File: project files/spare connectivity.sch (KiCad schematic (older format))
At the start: 2 parts, among them J6 Target STDC-14, U3 STM32F103CBUx

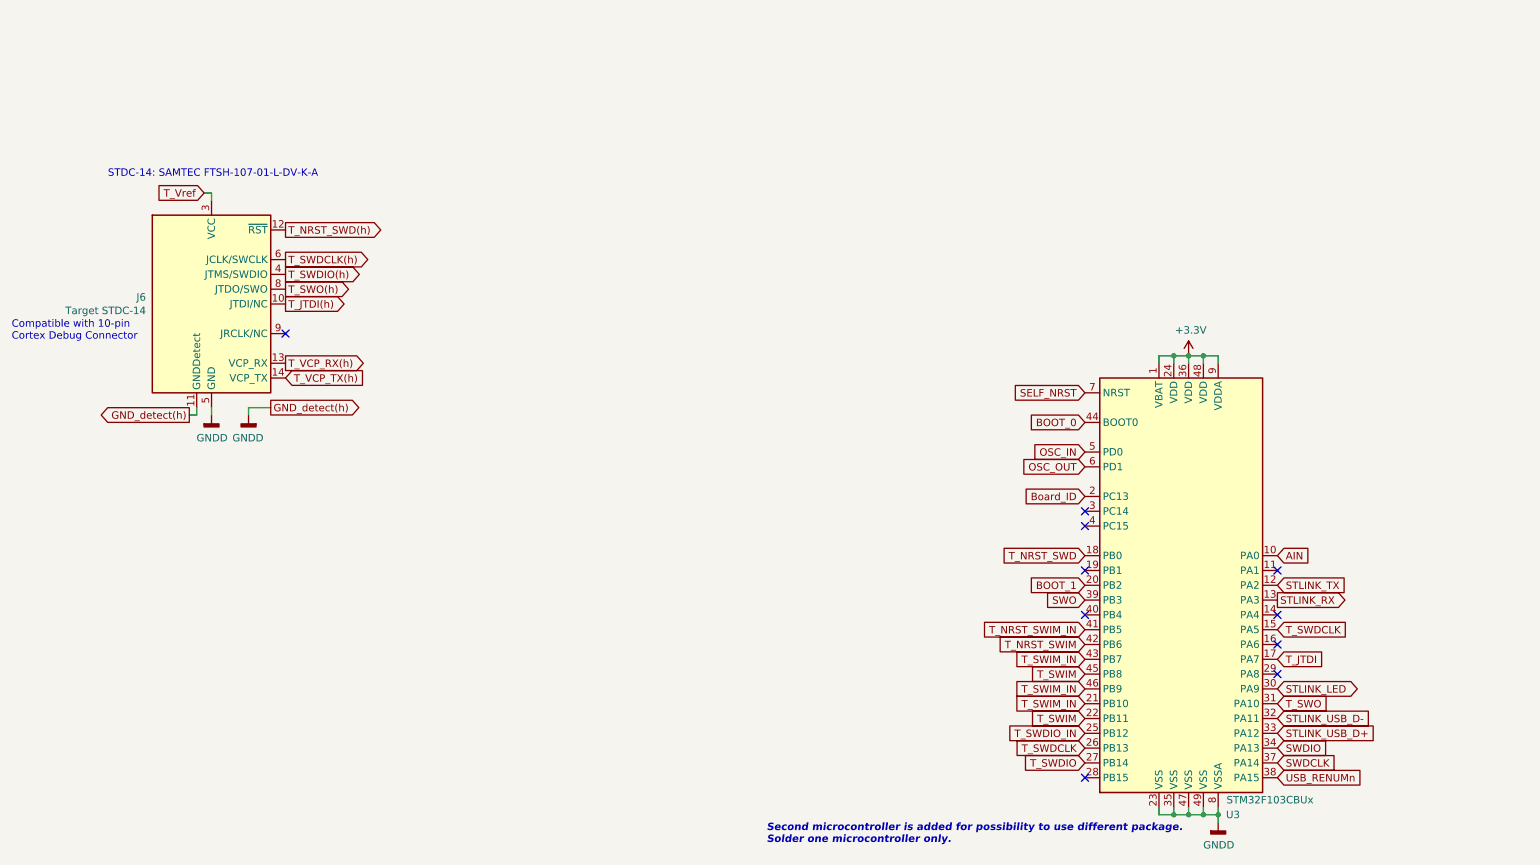
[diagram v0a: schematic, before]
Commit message: fixes
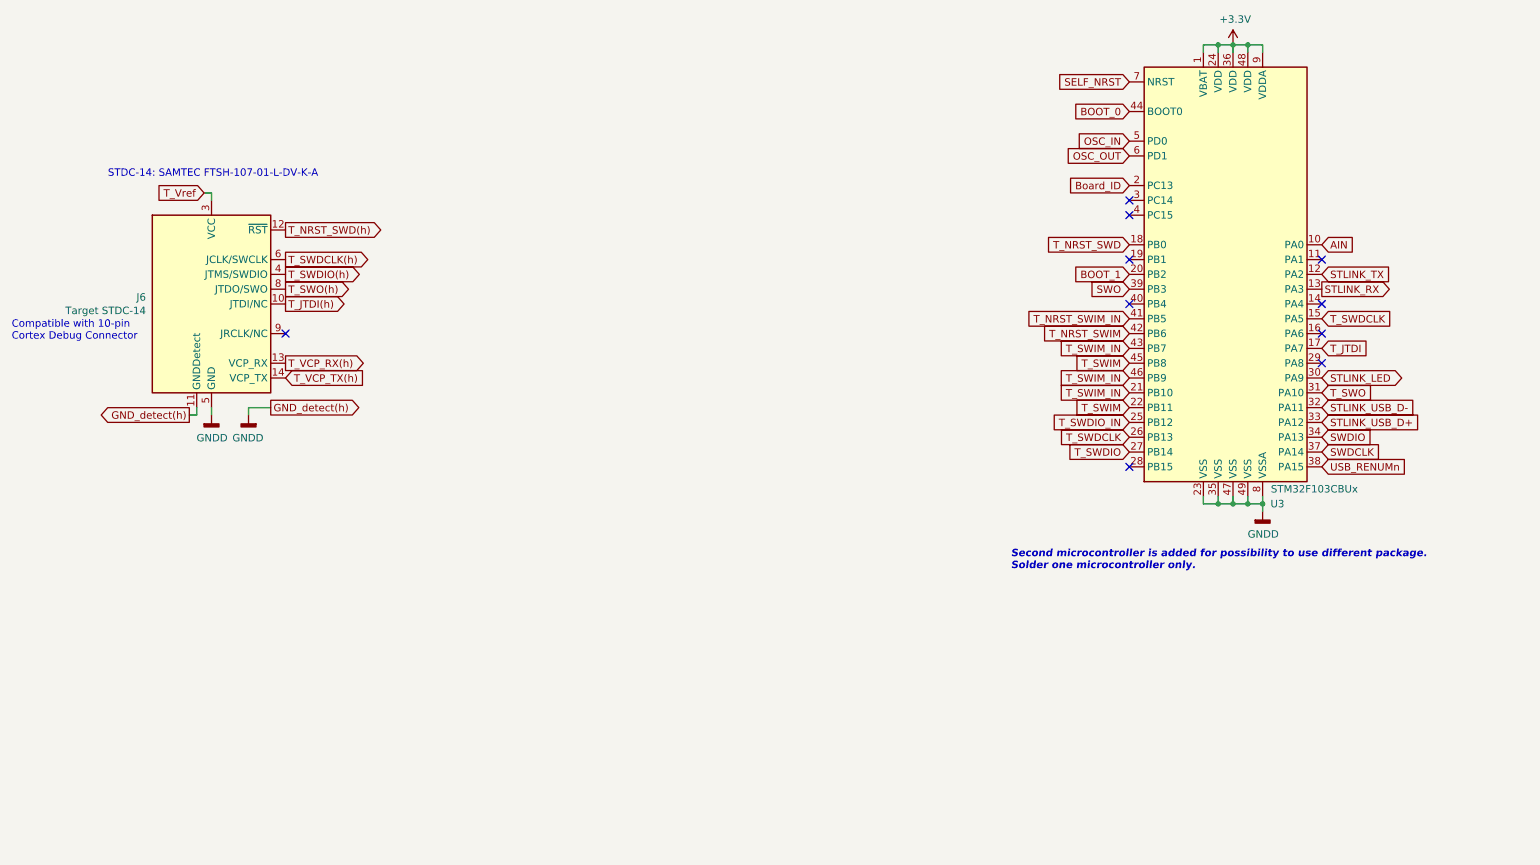
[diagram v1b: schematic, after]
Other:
- moved on the sheet: U3
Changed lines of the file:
@@
 Text Notes 2250 1800 0    50   ~ 0
 STDC-14: SAMTEC FTSH-107-01-L-DV-K-A
-Text GLabel 2800 3400 0    50   Output ~ 0
-GND_detect(h)
-Text GLabel 3350 3350 2    50   Output ~ 0
-GND_detect(h)
 $Comp
 L power:GNDD #PWR?
@@
 T_Vref
 Wire Wire Line
-	9750 6100 9750 6050
-Wire Wire Line
-	9650 6050 9650 6100
-Connection ~ 9650 6100
-Wire Wire Line
-	9650 6100 9750 6100
-Wire Wire Line
-	9550 6050 9550 6100
-Connection ~ 9550 6100
-Wire Wire Line
-	9550 6100 9650 6100
-Wire Wire Line
-	9450 6050 9450 6100
-Connection ~ 9450 6100
-Wire Wire Line
-	9450 6100 9550 6100
-Wire Wire Line
-	9350 6050 9350 6100
-Wire Wire Line
-	9350 6100 9450 6100
+	10050 4000 10050 3950
+Wire Wire Line
+	9950 3950 9950 4000
+Connection ~ 9950 4000
+Wire Wire Line
+	9950 4000 10050 4000
+Wire Wire Line
+	9850 3950 9850 4000
+Connection ~ 9850 4000
+Wire Wire Line
+	9850 4000 9950 4000
+Wire Wire Line
+	9750 3950 9750 4000
+Connection ~ 9750 4000
+Wire Wire Line
+	9750 4000 9850 4000
+Wire Wire Line
+	9650 3950 9650 4000
+Wire Wire Line
+	9650 4000 9750 4000
 $Comp
 L power:GNDD #PWR053
 U 1 1 5EC6BDFB
-P 9750 6150
-F 0 "#PWR053" H 9750 5900 50  0001 C CNN
-F 1 "GNDD" H 9754 5995 50  0000 C CNN
-F 2 "" H 9750 6150 50  0001 C CNN
-F 3 "" H 9750 6150 50  0001 C CNN
-	1    9750 6150
-	1    0    0    -1
-$EndComp
-Wire Wire Line
-	9750 6150 9750 6100
-Connection ~ 9750 6100
-Text Notes 6700 6300 0    50   Italic 10
+P 10050 4050
+F 0 "#PWR053" H 10050 3800 50  0001 C CNN
+F 1 "GNDD" H 10054 3895 50  0000 C CNN
+F 2 "" H 10050 4050 50  0001 C CNN
+F 3 "" H 10050 4050 50  0001 C CNN
+	1    10050 4050
+	1    0    0    -1
+$EndComp
+Wire Wire Line
+	10050 4050 10050 4000
+Connection ~ 10050 4000
+Text Notes 8350 4450 0    50   Italic 10
 Second microcontroller is added for possibility to use different package.\nSolder one microcontroller only.
-NoConn ~ 10150 5150
-NoConn ~ 10150 4950
-NoConn ~ 10150 4750
-NoConn ~ 10150 4450
-NoConn ~ 8850 5850
-NoConn ~ 8850 4750
-NoConn ~ 8850 4450
-NoConn ~ 8850 4150
-NoConn ~ 8850 4050
-Wire Wire Line
-	9350 3050 9350 3000
-Wire Wire Line
-	9450 3050 9450 3000
-Wire Wire Line
-	9550 3050 9550 3000
-Wire Wire Line
-	9650 3050 9650 3000
-Wire Wire Line
-	9750 3050 9750 3000
+NoConn ~ 10450 3050
+NoConn ~ 10450 2850
+NoConn ~ 10450 2650
+NoConn ~ 10450 2350
+NoConn ~ 9150 3750
+NoConn ~ 9150 2650
+NoConn ~ 9150 2350
+NoConn ~ 9150 2050
+NoConn ~ 9150 1950
+Wire Wire Line
+	9650 950  9650 900
+Wire Wire Line
+	9750 950  9750 900
+Wire Wire Line
+	9850 950  9850 900
+Wire Wire Line
+	9950 950  9950 900
+Wire Wire Line
+	10050 950  10050 900
 $Comp
 L MCU_ST_STM32F1:STM32F103CBUx U3
 U 1 1 5EC6BE12
-P 9550 4550
-F 0 "U3" H 9850 3000 50  0000 C CNN
-F 1 "STM32F103CBUx" H 10100 3100 50  0000 C CNN
-F 2 "Package_DFN_QFN:QFN-48-1EP_7x7mm_P0.5mm_EP5.6x5.6mm" H 8950 3150 50  0001 R CNN
-F 3 "http://www.st.com/st-web-ui/static/active/en/resource/technical/document/datasheet/CD00161566.pdf" H 9550 4550 50  0001 C CNN
-	1    9550 4550
-	1    0    0    -1
-$EndComp
-Text GLabel 10150 5250 2    50   BiDi ~ 0
+P 9850 2450
+F 0 "U3" H 10150 900 50  0000 C CNN
+F 1 "STM32F103CBUx" H 10400 1000 50  0000 C CNN
+F 2 "Package_DFN_QFN:QFN-48-1EP_7x7mm_P0.5mm_EP5.6x5.6mm" H 9250 1050 50  0001 R CNN
+F 3 "http://www.st.com/st-web-ui/static/active/en/resource/technical/document/datasheet/CD00161566.pdf" H 9850 2450 50  0001 C CNN
+	1    9850 2450
+	1    0    0    -1
+$EndComp
+Text GLabel 10450 3150 2    50   BiDi ~ 0
 STLINK_LED
-Text GLabel 8850 3650 0    50   Input ~ 0
+Text GLabel 9150 1550 0    50   Input ~ 0
 OSC_IN
-Text GLabel 8850 3750 0    50   Input ~ 0
+Text GLabel 9150 1650 0    50   Input ~ 0
 OSC_OUT
-Text GLabel 8850 3450 0    50   Input ~ 0
+Text GLabel 9150 1350 0    50   Input ~ 0
 BOOT_0
-Text GLabel 8850 3250 0    50   Input ~ 0
+Text GLabel 9150 1150 0    50   Input ~ 0
 SELF_NRST
-Text GLabel 8850 3950 0    50   Input ~ 0
+Text GLabel 9150 1850 0    50   Input ~ 0
 Board_ID
-Text GLabel 10150 4350 2    50   Input ~ 0
+Text GLabel 10450 2250 2    50   Input ~ 0
 AIN
-Text GLabel 10150 5450 2    50   Input ~ 0
+Text GLabel 10450 3350 2    50   Input ~ 0
 STLINK_USB_D-
-Text GLabel 10150 5550 2    50   Input ~ 0
+Text GLabel 10450 3450 2    50   Input ~ 0
 STLINK_USB_D+
-Text GLabel 10150 5350 2    50   Input ~ 0
+Text GLabel 10450 3250 2    50   Input ~ 0
 T_SWO
-Text GLabel 10150 5650 2    50   Input ~ 0
+Text GLabel 10450 3550 2    50   Input ~ 0
 SWDIO
-Text GLabel 10150 5750 2    50   Input ~ 0
+Text GLabel 10450 3650 2    50   Input ~ 0
 SWDCLK
-Text GLabel 10150 5850 2    50   Input ~ 0
+Text GLabel 10450 3750 2    50   Input ~ 0
 USB_RENUMn
-Text GLabel 8850 4650 0    50   Input ~ 0
+Text GLabel 9150 2550 0    50   Input ~ 0
 SWO
-Text GLabel 8850 4550 0    50   Input ~ 0
+Text GLabel 9150 2450 0    50   Input ~ 0
 BOOT_1
-Text GLabel 8850 5650 0    50   Input ~ 0
+Text GLabel 9150 3550 0    50   Input ~ 0
 T_SWDCLK
-Text GLabel 8850 4350 0    50   Input ~ 0
+Text GLabel 9150 2250 0    50   Input ~ 0
 T_NRST_SWD
-Text GLabel 8850 5350 0    50   Input ~ 0
+Text GLabel 9150 3250 0    50   Input ~ 0
 T_SWIM_IN
-Text GLabel 8850 5250 0    50   Input ~ 0
+Text GLabel 9150 3150 0    50   Input ~ 0
 T_SWIM_IN
-Text GLabel 8850 5050 0    50   Input ~ 0
+Text GLabel 9150 2950 0    50   Input ~ 0
 T_SWIM_IN
-Text GLabel 8850 4850 0    50   Input ~ 0
+Text GLabel 9150 2750 0    50   Input ~ 0
 T_NRST_SWIM_IN
-Text GLabel 8850 5750 0    50   Input ~ 0
+Text GLabel 9150 3650 0    50   Input ~ 0
 T_SWDIO
-Text GLabel 8850 4950 0    50   Input ~ 0
+Text GLabel 9150 2850 0    50   Input ~ 0
 T_NRST_SWIM
-Text GLabel 8850 5550 0    50   Input ~ 0
+Text GLabel 9150 3450 0    50   Input ~ 0
 T_SWDIO_IN
-Text GLabel 8850 5150 0    50   Input ~ 0
+Text GLabel 9150 3050 0    50   Input ~ 0
 T_SWIM
-Text GLabel 8850 5450 0    50   Input ~ 0
+Text GLabel 9150 3350 0    50   Input ~ 0
 T_SWIM
-Text GLabel 10150 4850 2    50   Input ~ 0
+Text GLabel 10450 2750 2    50   Input ~ 0
 T_SWDCLK
-Text GLabel 10150 4650 2    50   Output ~ 0
+Text GLabel 10450 2550 2    50   Output ~ 0
 STLINK_RX
-Text GLabel 10150 4550 2    50   Input ~ 0
+Text GLabel 10450 2450 2    50   Input ~ 0
 STLINK_TX
-Text GLabel 10150 5050 2    50   Input ~ 0
+Text GLabel 10450 2950 2    50   Input ~ 0
 T_JTDI
 Wire Wire Line
-	9350 3000 9450 3000
-Connection ~ 9450 3000
-Wire Wire Line
-	9450 3000 9550 3000
-Connection ~ 9550 3000
-Wire Wire Line
-	9550 3000 9650 3000
-Connection ~ 9650 3000
-Wire Wire Line
-	9650 3000 9750 3000
+	9650 900  9750 900
+Connection ~ 9750 900
+Wire Wire Line
+	9750 900  9850 900
+Connection ~ 9850 900
+Wire Wire Line
+	9850 900  9950 900
+Connection ~ 9950 900
+Wire Wire Line
+	9950 900  10050 900
 $Comp
 L power:+3.3V #PWR052
 U 1 1 5EC6FD9F
-P 9550 3000
-F 0 "#PWR052" H 9550 2850 50  0001 C CNN
-F 1 "+3.3V" H 9565 3173 50  0000 C CNN
-F 2 "" H 9550 3000 50  0001 C CNN
-F 3 "" H 9550 3000 50  0001 C CNN
-	1    9550 3000
-	1    0    0    -1
-$EndComp
+P 9850 900
+F 0 "#PWR052" H 9850 750 50  0001 C CNN
+F 1 "+3.3V" H 9865 1073 50  0000 C CNN
+F 2 "" H 9850 900 50  0001 C CNN
+F 3 "" H 9850 900 50  0001 C CNN
+	1    9850 900
+	1    0    0    -1
+$EndComp
+Text GLabel 3350 3350 2    50   Output ~ 0
+GND_detect(h)
+Text GLabel 2800 3400 0    50   Output ~ 0
+GND_detect(h)
 $EndSCHEMATC
